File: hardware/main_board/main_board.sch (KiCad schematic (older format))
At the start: 34 parts, among them P2 CONN_01X02, SW1 SW_DPDT_x2, SW2 SW_Push, U1 ESP-12E, U3 MCP9808, U4 MMA8451Q, U5 MCP73831/2, U6 AP2112

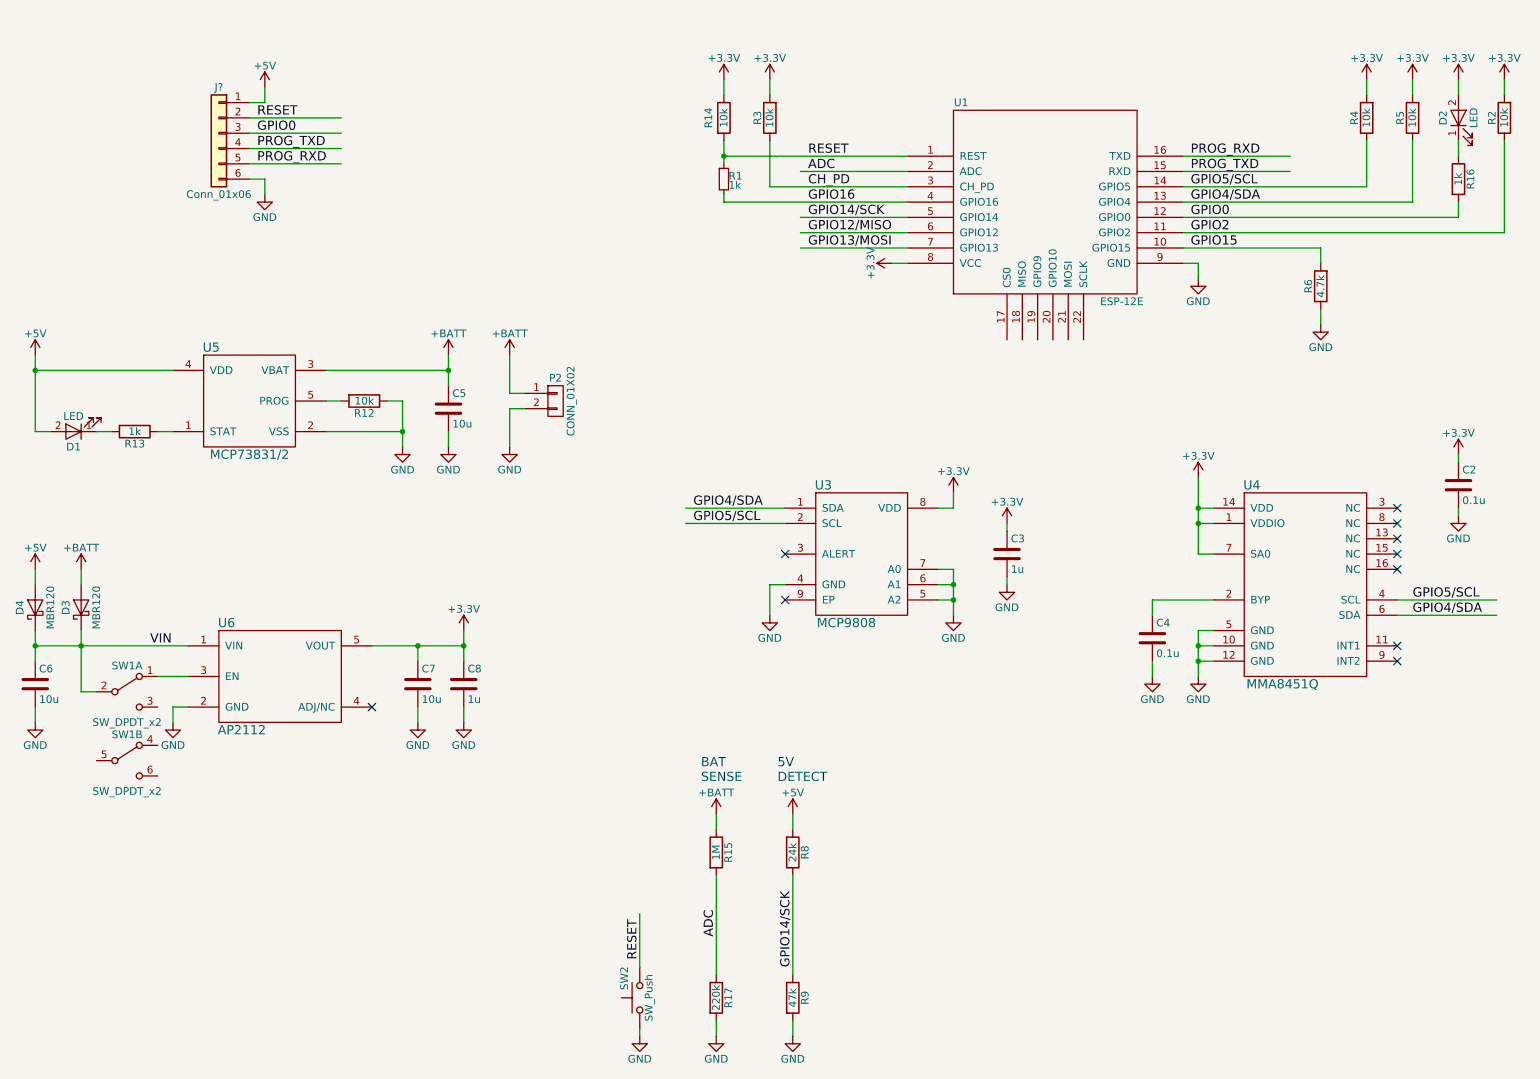
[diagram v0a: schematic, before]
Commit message: Working on schematic
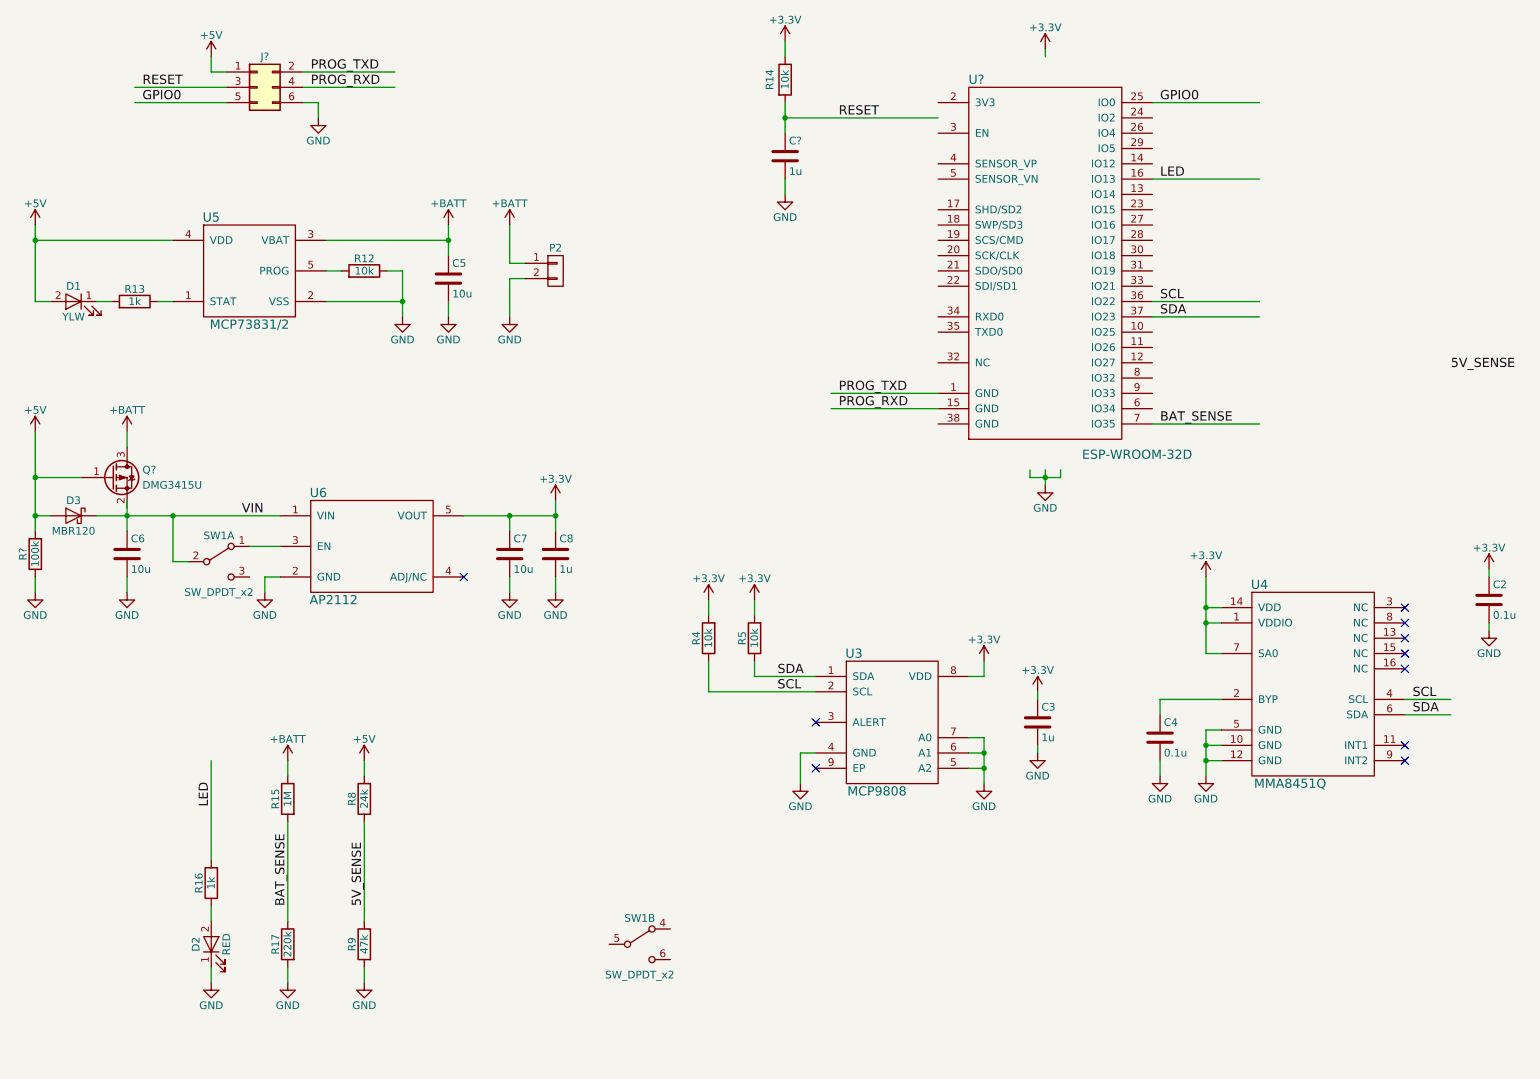
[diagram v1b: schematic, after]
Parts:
- removed D4: MBR120, footprint:SOD-123FL, symbol D_Schottky
- removed J?: Conn_01x06, symbol Conn_01x06
- removed R1: 1k, Resistors_SMD:R_0603, symbol R_Small
- removed R2, R3: 10k, Resistors_SMD:R_0603, symbol R
- removed R6: 4.7k, Resistors_SMD:R_0603, symbol R
- removed SW2: SW_Push, footprint:KMR7, symbol SW_Push
- removed U1: ESP-12E, footprint:ESP-12E, symbol ESP-12E
- added C?: 1u, Capacitors_SMD:C_0603, symbol C
- added J?: eConn_02x03_Odd_Even, symbol Conn_02x03_Odd_Even
- added Q?: DMG3415U, TO_SOT_Packages_SMD:SOT-23, symbol Q_PMOS_GSD
- added R?: 100k, Resistors_SMD:R_0603, symbol R
- added U?: ESP-WROOM-32D, symbol ESP-WROOM-32D
- D1: value LED -> YLW
- D2: value LED -> RED
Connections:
- net labels added: 5V_SENSE, BAT_SENSE, LED, SCL, SDA
- net labels removed: ADC, CH_PD, GPIO12/MISO, GPIO13/MOSI, GPIO14/SCK, GPIO15, GPIO16, GPIO2, GPIO4/SDA, GPIO5/SCL
- wire segments 107 -> 98
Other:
- note removed: "5V\nDETECT"
- note removed: "BAT\nSENSE"
- moved on the sheet: C2, C3, C4, C5, C6, C7, C8, D1, D2, D3, P2, R12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
